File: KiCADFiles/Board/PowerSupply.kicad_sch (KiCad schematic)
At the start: 30 parts, among them J3 Barrel_Jack_PTH, U2 LT1962-3.3, U3 LT1962-5, U8 LT1962

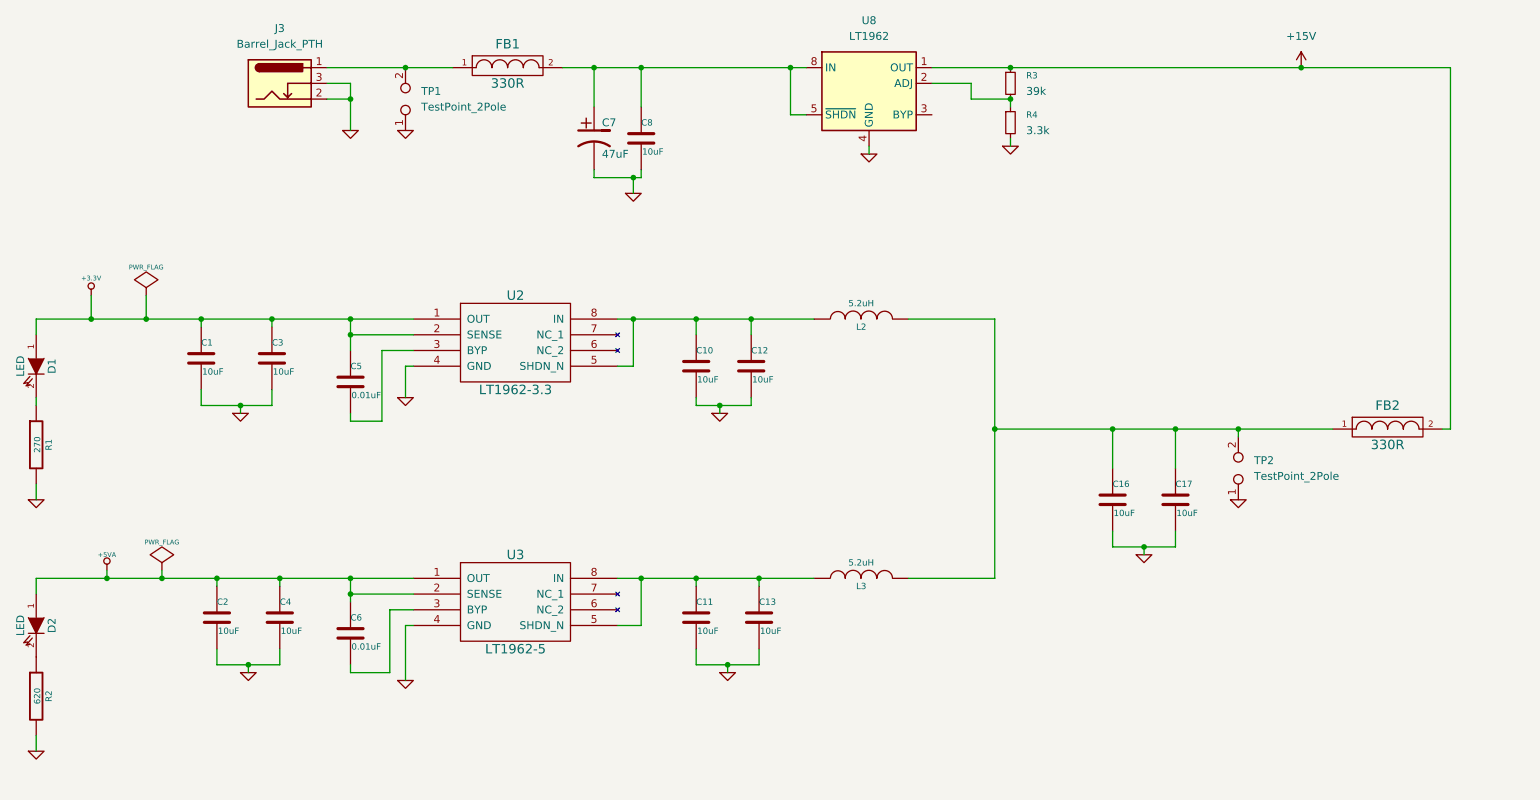
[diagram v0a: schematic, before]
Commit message: chose all components
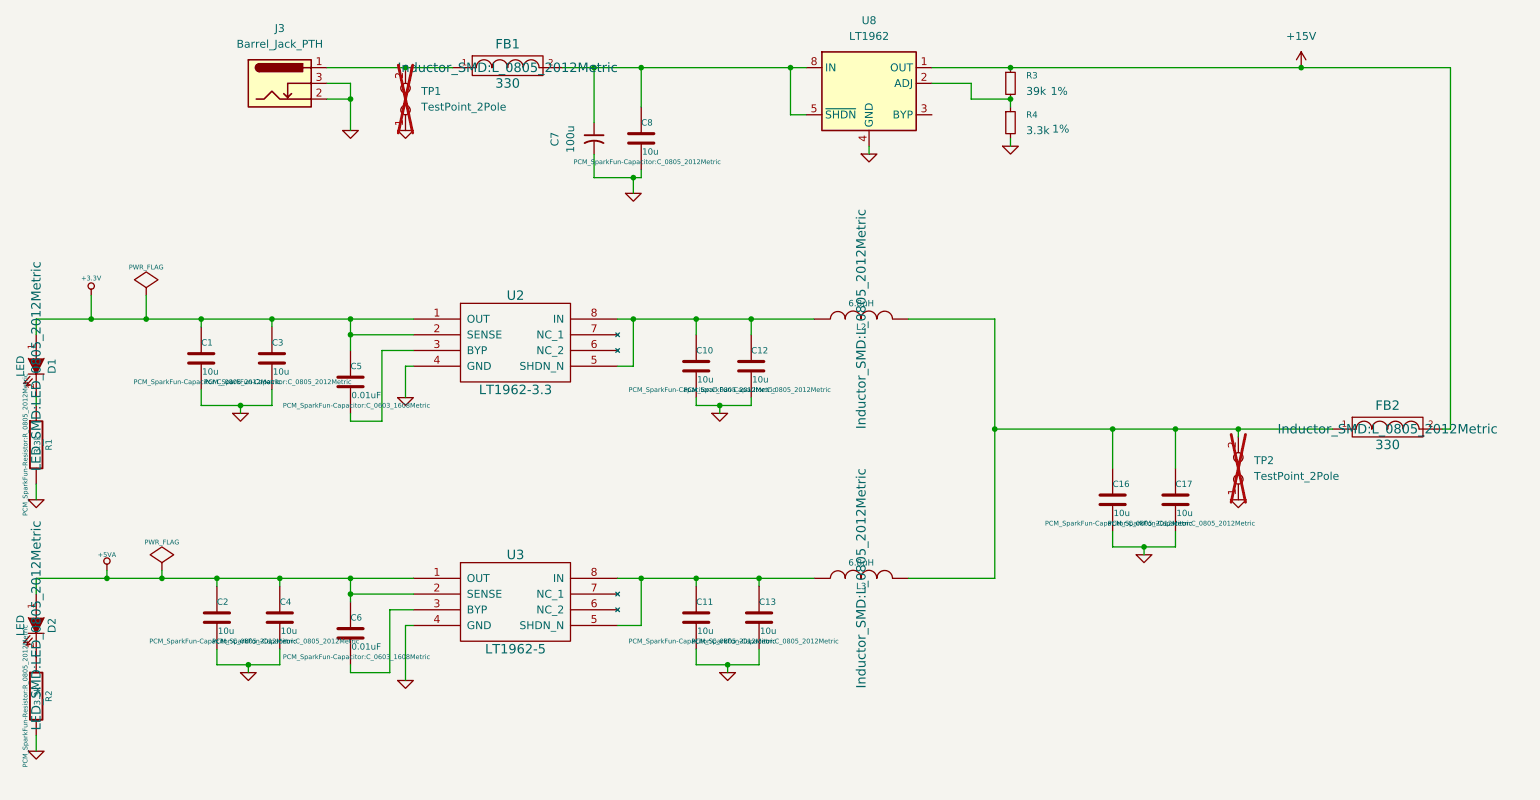
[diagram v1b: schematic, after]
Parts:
- removed C7: 47uF, ~, symbol SuperAudioBoard-rescue:CP1
- added C7: 100u, Capacitor_THT:CP_Radial_D5.0mm_P2.00mm, symbol Device:C_Small_US
- C1, C10, C11, C12, C13, C16, C17, C2, C3, C4, C8: value 10uF -> 10u; footprint ~ -> PCM_SparkFun-Capacitor:C_0805_2012Metric; MPN (none) -> CL21A106KAYNNNG; Voltage (none) -> 25V
- C5, C6: footprint ~ -> PCM_SparkFun-Capacitor:C_0603_1608Metric; MPN (none) -> C0603C103K5RACTU
- D1, D2: footprint ~ -> LED_SMD:LED_0805_2012Metric; MPN (none) -> 599-0110-137F
- FB1, FB2: value 330R -> 330; footprint ~ -> Inductor_SMD:L_0805_2012Metric; MPN (none) -> MPZ2012S331ATD25
- L2, L3: value 5.2uH -> 6.8uH; footprint ~ -> Inductor_SMD:L_0805_2012Metric; MPN (none) -> MLZ2012N6R8LT000
- R1: value 270 -> 3.3k; footprint ~ -> PCM_SparkFun-Resistor:R_0805_2012Metric; MPN (none) -> ERA-6AEB332V
- R2: value 620 -> 3.3k; footprint ~ -> PCM_SparkFun-Resistor:R_0805_2012Metric; MPN (none) -> ERA-6AEB332V
- R3: footprint (none) -> PCM_SparkFun-Resistor:R_0805_2012Metric; MPN (none) -> ERA-6AEB3922V; Tol (none) -> 1%
- R4: footprint (none) -> PCM_SparkFun-Resistor:R_0805_2012Metric; MPN (none) -> ERA-6AEB332V; Tol (none) -> 1%
- TP1, TP2: footprint (none) -> TestPoint:TestPoint_2Pads_Pitch2.54mm_Drill0.8mm; now not fitted
- U2: footprint (none) -> Package_SO:MSOP-8_3x3mm_P0.65mm; MPN (none) -> LT1962EMS8-3.3
- U3: footprint (none) -> Package_SO:MSOP-8_3x3mm_P0.65mm; MPN (none) -> LT1962EMS8-5
- U8: MPN (none) -> LT1962EMS8
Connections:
- net GND: now also C7.2
- net at C8.1, FB1.2, U8.5 (~{SHDN})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: now also C7.1
